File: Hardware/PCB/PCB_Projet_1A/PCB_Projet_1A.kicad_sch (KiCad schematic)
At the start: 19 parts, among them J1 Conn_01x03, J13 Conn_01x06, J2 Conn_01x04, J3 Conn_01x03, J4 Conn_01x04, J5 Conn_01x04, J6 Conn_ST_STDC14, J7 Conn_01x04, J8 Conn_01x02, J9 Conn_01x02

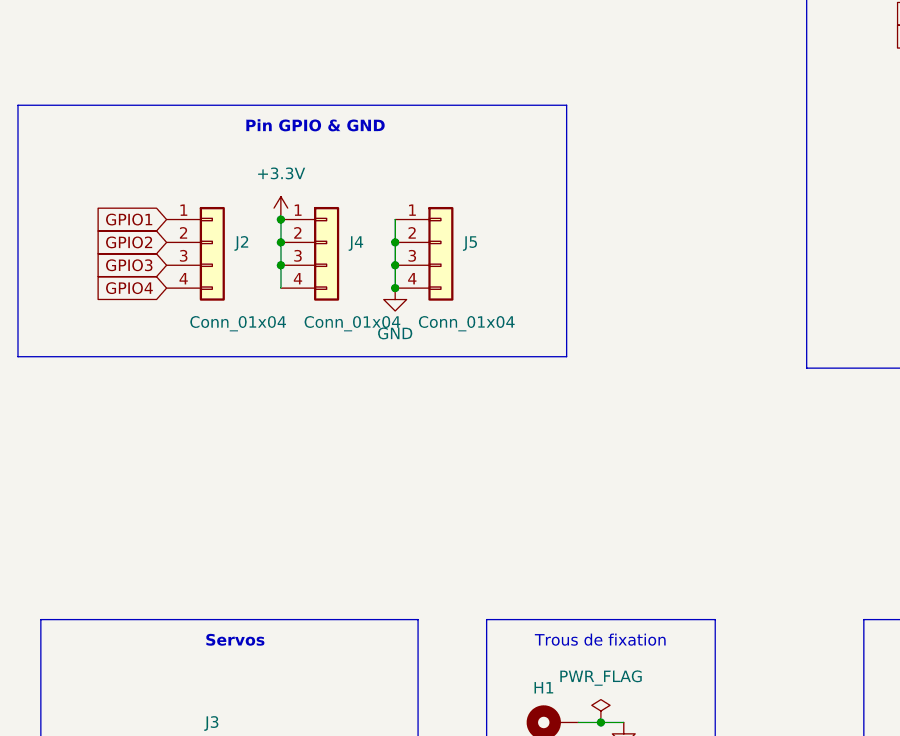
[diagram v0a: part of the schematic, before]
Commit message: modif pcb
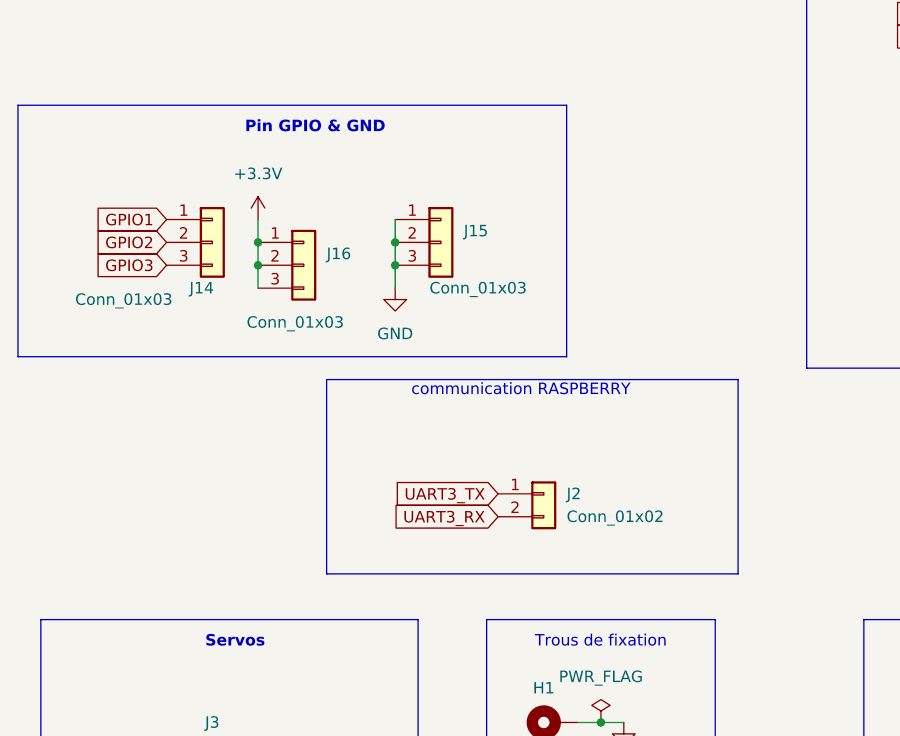
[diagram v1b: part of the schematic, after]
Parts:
- removed J2, J4, J5: Conn_01x04, Connector_PinHeader_2.54mm:PinHeader_1x04_P2.54mm_Vertical, symbol Connector_Generic:Conn_01x04
- added J14, J15, J16: Conn_01x03, Connector_PinHeader_2.54mm:PinHeader_1x03_P2.54mm_Vertical, symbol Connector_Generic:Conn_01x03
- added J2: Conn_01x02, Connector_PinHeader_2.54mm:PinHeader_1x02_P2.54mm_Horizontal, symbol Connector_Generic:Conn_01x02
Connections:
- net +3.3V: now also J16.1 (Pin_1), J16.2 (Pin_2), J16.3 (Pin_3)
- net GND: now also J15.1 (Pin_1), J15.2 (Pin_2), J15.3 (Pin_3)
- net GPIO1: now also J14.1 (Pin_1)
- net GPIO2: now also J14.2 (Pin_2)
- net GPIO3: now also J14.3 (Pin_3)
- new net UART3_RX: J2.2 (Pin_2)
- new net UART3_TX: J2.1 (Pin_1)
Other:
- note added: "communication RASPBERRY"
